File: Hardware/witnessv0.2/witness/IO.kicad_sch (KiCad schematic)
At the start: 14 parts, among them J2 Conn_01x02, J3 USB_B_Micro, J5 Conn_01x04, J6 Conn_01x04, U5 TCAN1044A-Q1, U9 USBLC6-2SC6

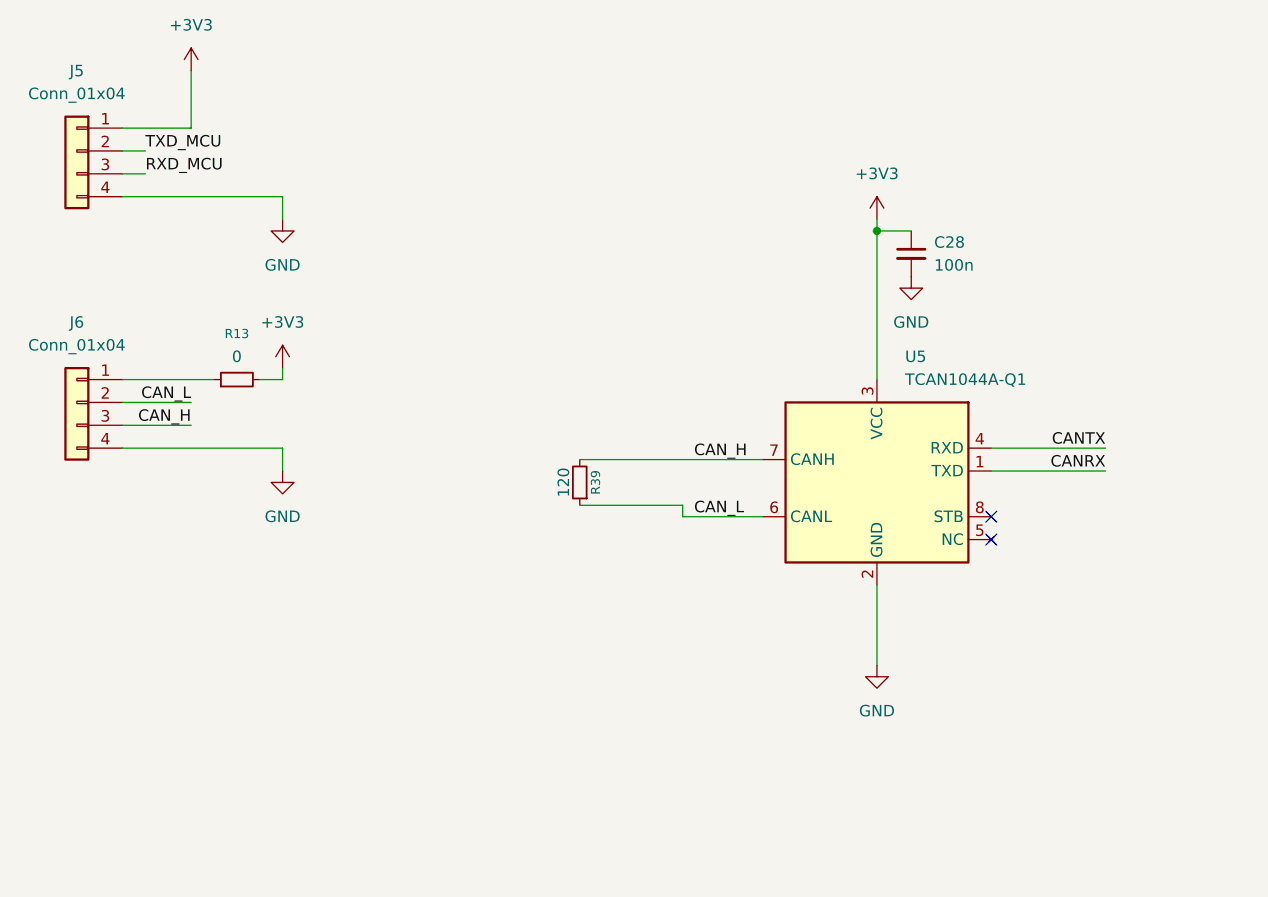
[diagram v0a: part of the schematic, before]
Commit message: root feedback
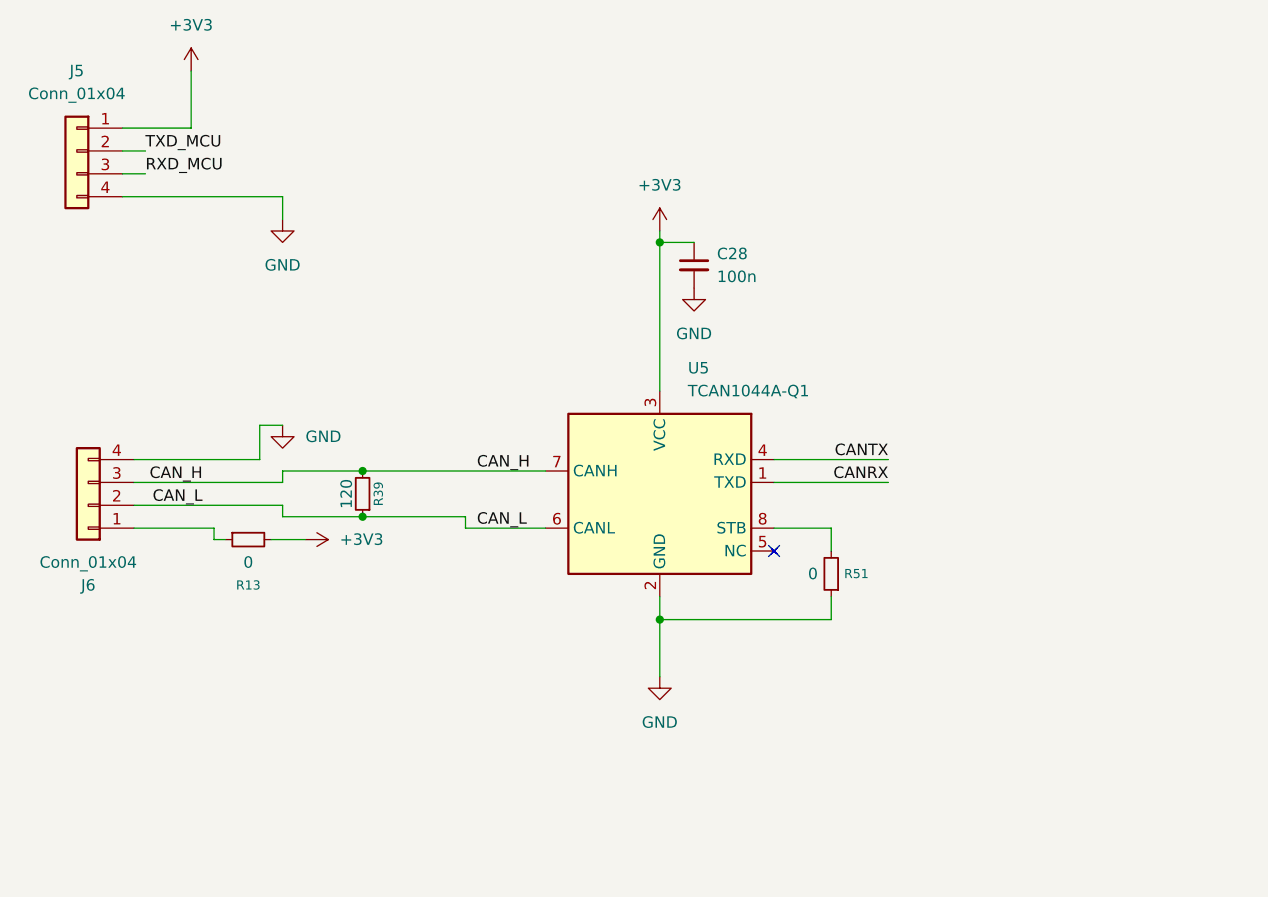
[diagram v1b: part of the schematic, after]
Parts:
- added R51: 0, Resistor_SMD:R_0402_1005Metric, symbol Device:R_Small
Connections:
- net GND: now also R51.1
- net at U5.8 (STB): now also R51.2
- no-connect marks 3 -> 2
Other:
- moved on the sheet: C28, J6, R13, R39, U5

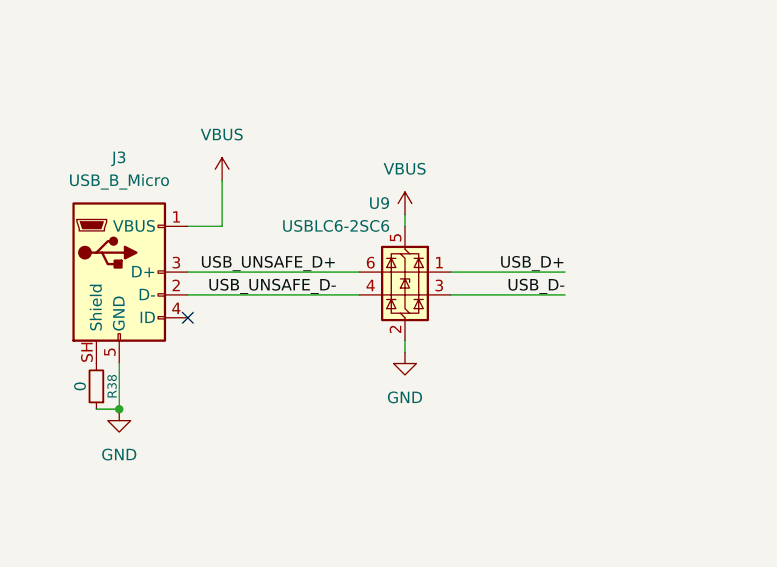
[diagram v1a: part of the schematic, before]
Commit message: updates from folks
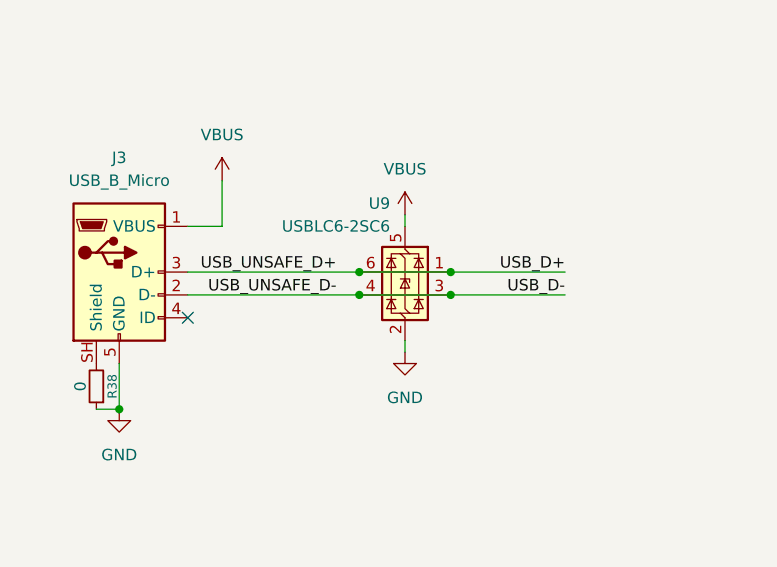
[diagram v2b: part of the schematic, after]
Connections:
- net USB_UNSAFE_D+ is gone; now on net USB_D+: J3.3 (D+), U9.6 (I/O1)
- net USB_UNSAFE_D- is gone; now on net USB_D-: J3.2 (D-), U9.4 (I/O2)
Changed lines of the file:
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@@
+	)
+	(junction
+		(at 240.03 121.92)
+		(diameter 0)
+		(color 0 0 0 0)
+	)
+	(junction
+		(at 240.03 124.46)
+		(diameter 0)
+		(color 0 0 0 0)
 	)
 	(junction
@@
 	)
 	(junction
+		(at 250.19 124.46)
+		(diameter 0)
+		(color 0 0 0 0)
+	)
+	(junction
 		(at 68.58 93.98)
+		(diameter 0)
+		(color 0 0 0 0)
+	)
+	(junction
+		(at 250.19 121.92)
 		(diameter 0)
 		(color 0 0 0 0)
@@
 	(wire
 		(pts
+			(xy 240.03 121.92) (xy 250.19 121.92)
+		)
+		(stroke
+			(width 0)
+			(type default)
+		)
+	)
+	(wire
+		(pts
 			(xy 135.89 162.56) (xy 139.7 162.56)
 		)
@@
 		)
 		(stroke
+			(width 0)
+			(type default)
+		)
+	)
+	(wire
+		(pts
+			(xy 240.03 124.46) (xy 250.19 124.46)
+		)
+		(stroke
